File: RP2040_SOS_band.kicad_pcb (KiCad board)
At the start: 4 copper layers, 127 x 67.9 mm, 87 parts, among them J1 TYPE_C-31M12, J2 SIM8060-6-0-14-00-A, J3 10Pin FPC TOP Board, J4 10Pin FPC Bottom board, J5 U.FL-R-SMT-1(10), Q1 HSSN3134, SW1 Boot, SW2 PWR, SW3 NAV, U1 RP2040, U10 M66, U2 TPS7A7001DDA, U3 W25Q32JVSS, U4 MAX30102, U5 MCP73831-2-OT, U6 MPU-6050, U7 AZ1117-1.8, U8 L96, Y1 Crystal_GND24

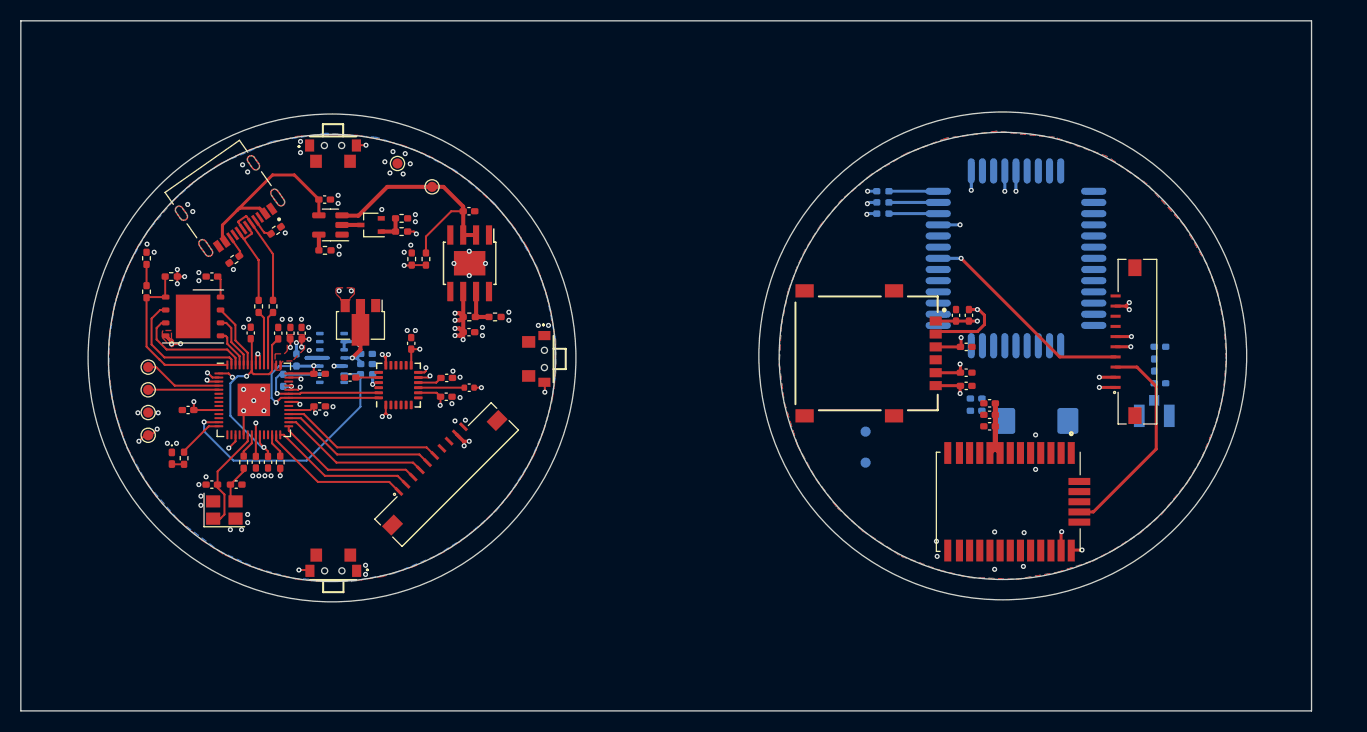
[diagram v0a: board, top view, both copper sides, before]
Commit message: Final Design
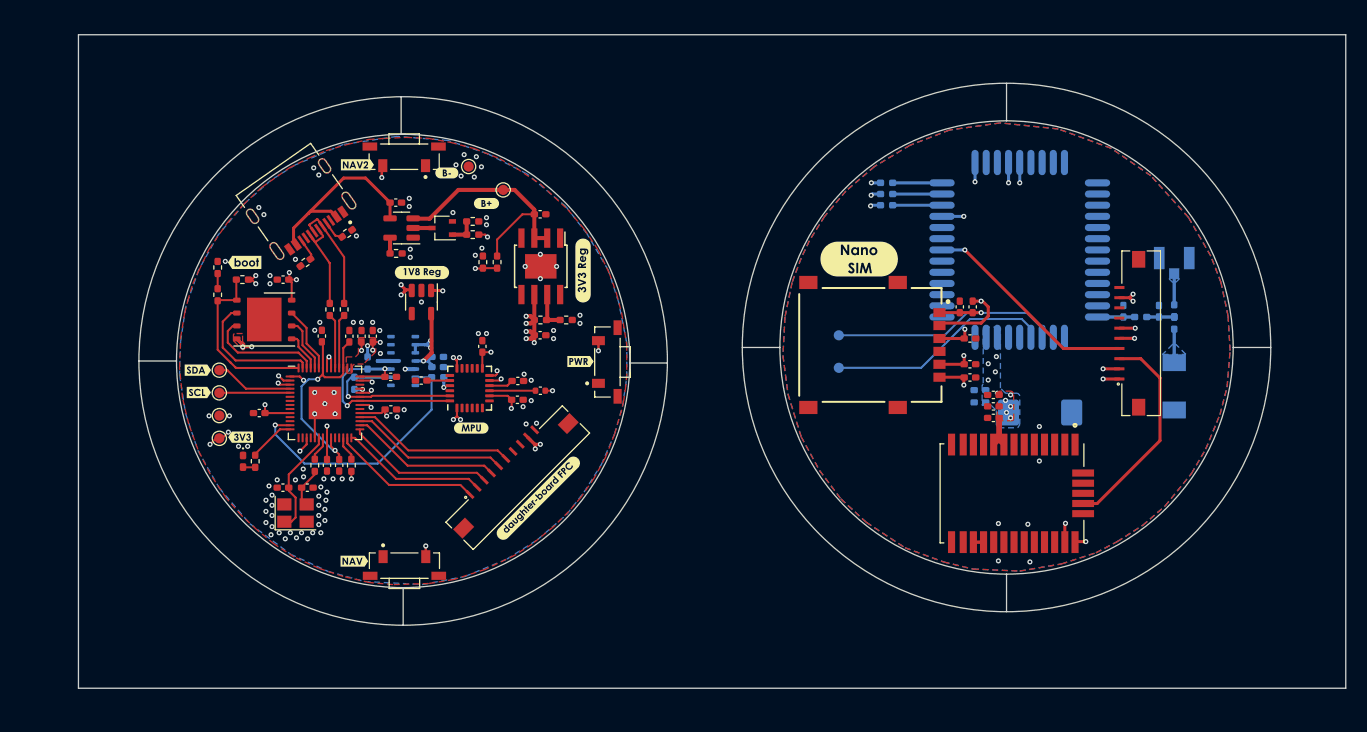
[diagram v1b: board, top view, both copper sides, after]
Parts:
- added E1: NN02-201, NN02-201:XCVR_NN02-201, B.Cu at (198.0, 92.9)
- added R12: 0, Resistor_SMD:R_0402_1005Metric_Pad0.72x0.64mm_HandSolder, B.Cu at (198.0, 85.4)
- added R24: 0, Resistor_SMD:R_0402_1005Metric_Pad0.72x0.64mm_HandSolder, B.Cu at (198.0, 86.6)
- added kibuzzard-648D8F43: G***, kibuzzard-648D8F43, F.Cu at (106.1, 97.9)
- added kibuzzard-648D8F93: G***, kibuzzard-648D8F93, F.Cu at (139.6, 90.4)
- added kibuzzard-648D8FB3: G***, kibuzzard-648D8FB3, F.Cu at (117.3, 110.1)
- added kibuzzard-648D8FC5: G***, kibuzzard-648D8FC5, F.Cu at (117.6, 71.1)
- added kibuzzard-648D902E: G***, kibuzzard-648D902E, F.Cu at (128.8, 97.0)
- added kibuzzard-648D909E: G***, kibuzzard-648D909E, F.Cu at (106.5, 80.7)
- added kibuzzard-648D90C6: G***, kibuzzard-648D90C6, F.Cu at (139.8, 81.5)
- added kibuzzard-648D90E2: G***, kibuzzard-648D90E2, F.Cu at (124.0, 81.7)
- added kibuzzard-648D9126: G***, kibuzzard-648D9126, B.Cu at (123.0, 86.4)
- added kibuzzard-648D91AF: G***, kibuzzard-648D91AF, F.Cu at (135.4, 103.9)
- added kibuzzard-648D920B: G***, kibuzzard-648D920B, F.Cu at (130.3, 74.9)
- added kibuzzard-648D921A: G***, kibuzzard-648D921A, F.Cu at (126.4, 71.9)
- added kibuzzard-648D92FA: G***, kibuzzard-648D92FA, F.Cu at (167.0, 80.3)
- added kibuzzard-648D9334: G***, kibuzzard-648D9334, B.Cu at (165.0, 94.3)
- added kibuzzard-648D9374: G***, kibuzzard-648D9374, B.Cu at (165.0, 84.4)
- added kibuzzard-648D9446: G***, kibuzzard-648D9446, F.Cu at (101.9, 91.3)
- added kibuzzard-648D944C: G***, kibuzzard-648D944C, F.Cu at (102.0, 93.5)
- Q1: value HSSN3134 -> BSS214
- SW1: value Boot -> NAV2; footprint TS24CA Tactile switch:TS24CA -> TL3330AF260QG:SW_TL3330AF260QG
- SW2, SW3: footprint TS24CA Tactile switch:TS24CA -> TL3330AF260QG:SW_TL3330AF260QG
- U7: value AZ1117-1.8 -> AP2127K-1.8; footprint Package_TO_SOT_SMD:SOT-89-3 -> Package_TO_SOT_SMD:SOT-23-5
- moved J5 15.7 mm to (198.0, 80.2), turned to 180 degrees
- moved TP1 12.8 mm to (165.0, 87.8)
- moved C33 7.96 mm to (193.0, 85.5), turned to 90 degrees
- moved SW1 7.09 mm to (122.2, 70.3), turned to 180 degrees
- moved R11 7.06 mm to (103.9, 81.2)
- moved SW3 7.02 mm to (122.2, 110.5), turned to 0 degrees
- moved C1 7.01 mm to (108.0, 95.5)
- moved C12 7.01 mm to (110.3, 82.4)
- moved C13 7.01 mm to (110.3, 102.8)
- moved C14 7.01 mm to (112.7, 102.8)
- moved C17 7.01 mm to (123.9, 92.3)
- moved C18 7.01 mm to (133.4, 94.2)
- moved C19 7.01 mm to (133.4, 92.3)
- moved C2 7.01 mm to (120.9, 91.9)
- moved C20 7.01 mm to (125.5, 90.0)
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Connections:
- C32 pad 1: Net-(J5-SIG) -> Net-(C32-Pad1)
- R23 pad 2: Net-(J5-SIG) -> Net-(C32-Pad1)
- U7 pad 1: GND -> VDD_3.3
- U7 pad 2: +1V8 -> GND
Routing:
- net Net-(U10-DBG_RXD): track 0.00 -> 22.4 mm
- net Net-(U10-DBG_TXD): track 0.00 -> 22.2 mm
- net NAV_BUTTON_2: track 31.1 -> 26.2 mm
- net VDD_3.3: track 50.1 -> 54.4 mm, vias 32 -> 34
- net Net-(U10-RF_ANT): track 0.00 -> 3.65 mm
- net Net-(E1-Pad1): track 0.00 -> 3.30 mm
- net Net-(J5-SIG): track 0.00 -> 3.08 mm
- net Net-(C32-Pad1): track 0.00 -> 2.70 mm
- net VDD_3.3_t: track 9.92 -> 7.65 mm, vias 3 -> 12
- net NAV_BUTTON: track 17.6 -> 19.1 mm
- net PWR_BUTTON: track 40.2 -> 41.3 mm
- net Net-(U8-RF_IN): track 0.00 -> 1.00 mm
- net Net-(R11-Pad2): track 2.09 -> 1.49 mm
- net GND: vias 92 -> 106
- added copper zone on B.Cu, net Net-(E1-Pad1)
- added copper zone on B.Cu, net Net-(J5-SIG)
- added copper zone on B.Cu, net VDD_3.3_t
- added copper zone on F.Cu, net VDD_3.3_t
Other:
- board size 127 x 67.9 mm -> 124.7 x 64.3 mm
